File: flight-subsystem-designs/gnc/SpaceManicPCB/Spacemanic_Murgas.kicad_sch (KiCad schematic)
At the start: 1 part

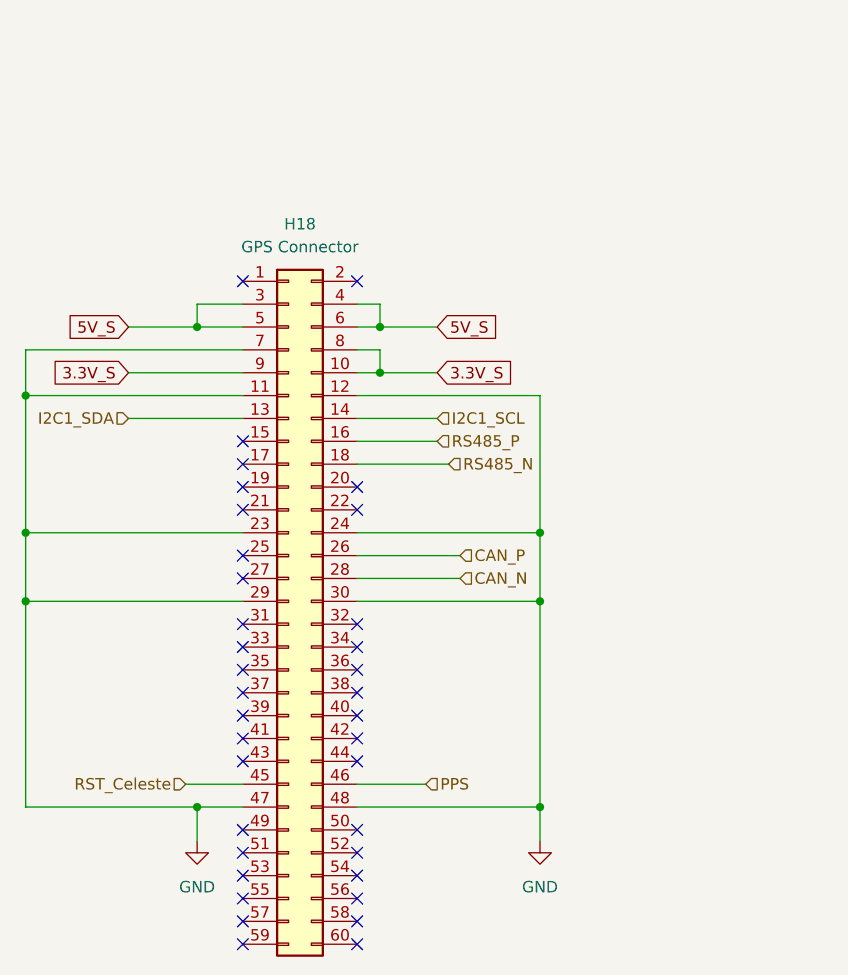
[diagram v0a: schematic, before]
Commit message: Final Changes
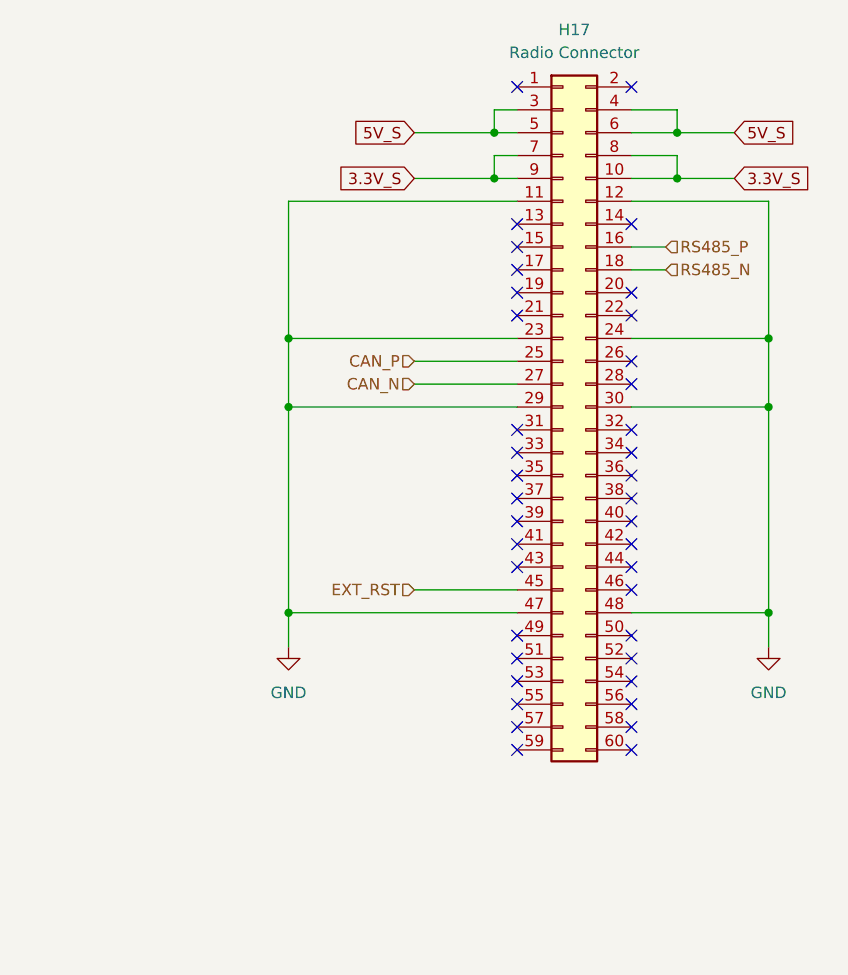
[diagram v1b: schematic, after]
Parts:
- removed H18: GPS Connector, Connector_Molex:CON_MolexSlimStack_54363-0689, symbol Connector_Generic:Conn_02x30_Odd_Even
- added H17: Radio Connector, Connector_Molex:CON_MolexSlimStack_54363-0689, symbol Connector_Generic:Conn_02x30_Odd_Even
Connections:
- net 3.3V_S: now also H17.10 (Pin_10), H17.7 (Pin_7), H17.8 (Pin_8), H17.9 (Pin_9)
- net 5V_S: now also H17.3 (Pin_3), H17.4 (Pin_4), H17.5 (Pin_5), H17.6 (Pin_6)
- net CAN_N: now also H17.27 (Pin_27)
- net CAN_P: now also H17.25 (Pin_25)
- net GND: now also H17.11 (Pin_11), H17.12 (Pin_12), H17.23 (Pin_23), H17.24 (Pin_24), H17.29 (Pin_29), H17.30 (Pin_30), H17.47 (Pin_47), H17.48 (Pin_48)
- net RS485_N: now also H17.18 (Pin_18)
- net RS485_P: now also H17.16 (Pin_16)
- new net EXT_RST: H17.45 (Pin_45)
- no-connect marks 36 -> 39
